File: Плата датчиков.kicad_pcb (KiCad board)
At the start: 4 copper layers, 67 x 68.5 mm, 57 parts, among them J1 A, J10 4900, J11 4900, J12 4900, J13 4900, J14 4900, J2 B, J3 C, J4 Conn_02x07_Odd_Even, J5 4900, J6 4900, J7 4900, J8 Conn_02x02_Odd_Even, J9 4900, U1 INA282, U2 INA282, U3 INA282, U4 LMV324

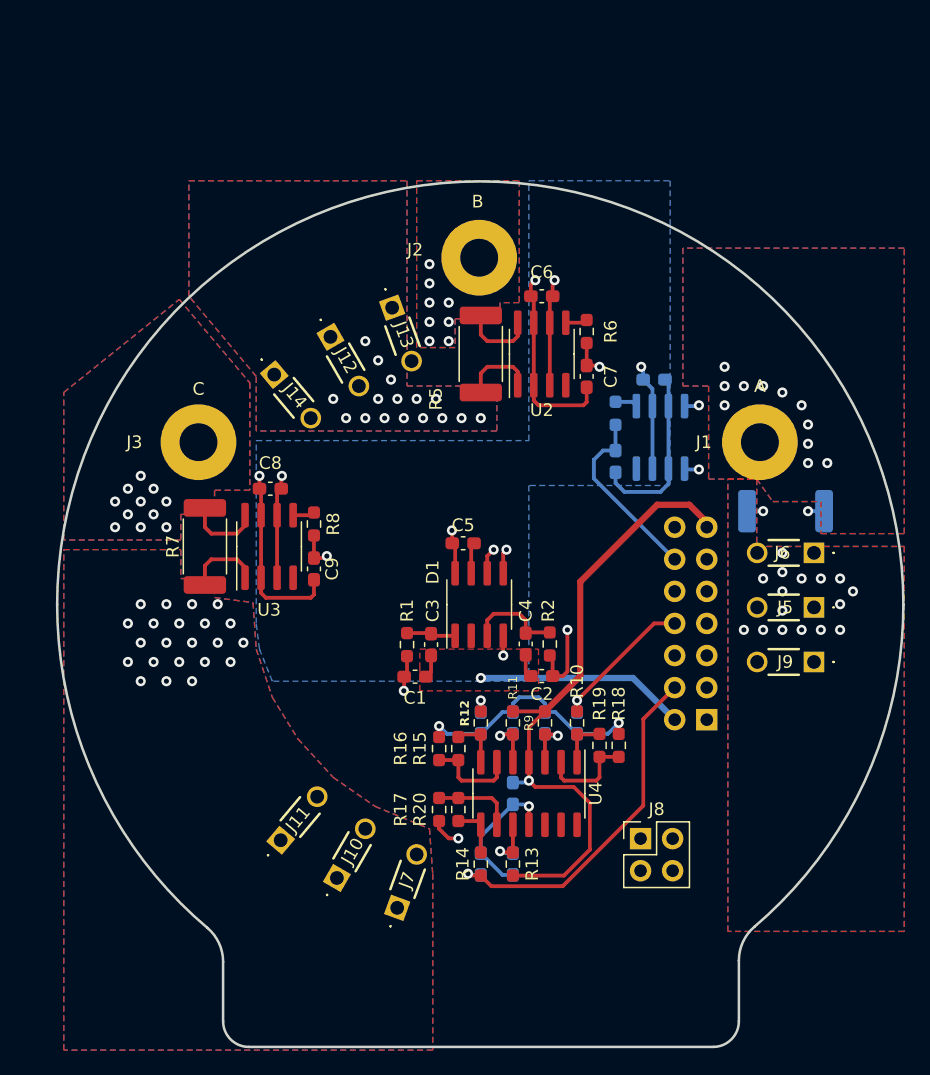
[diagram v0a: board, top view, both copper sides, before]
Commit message: VER2.0
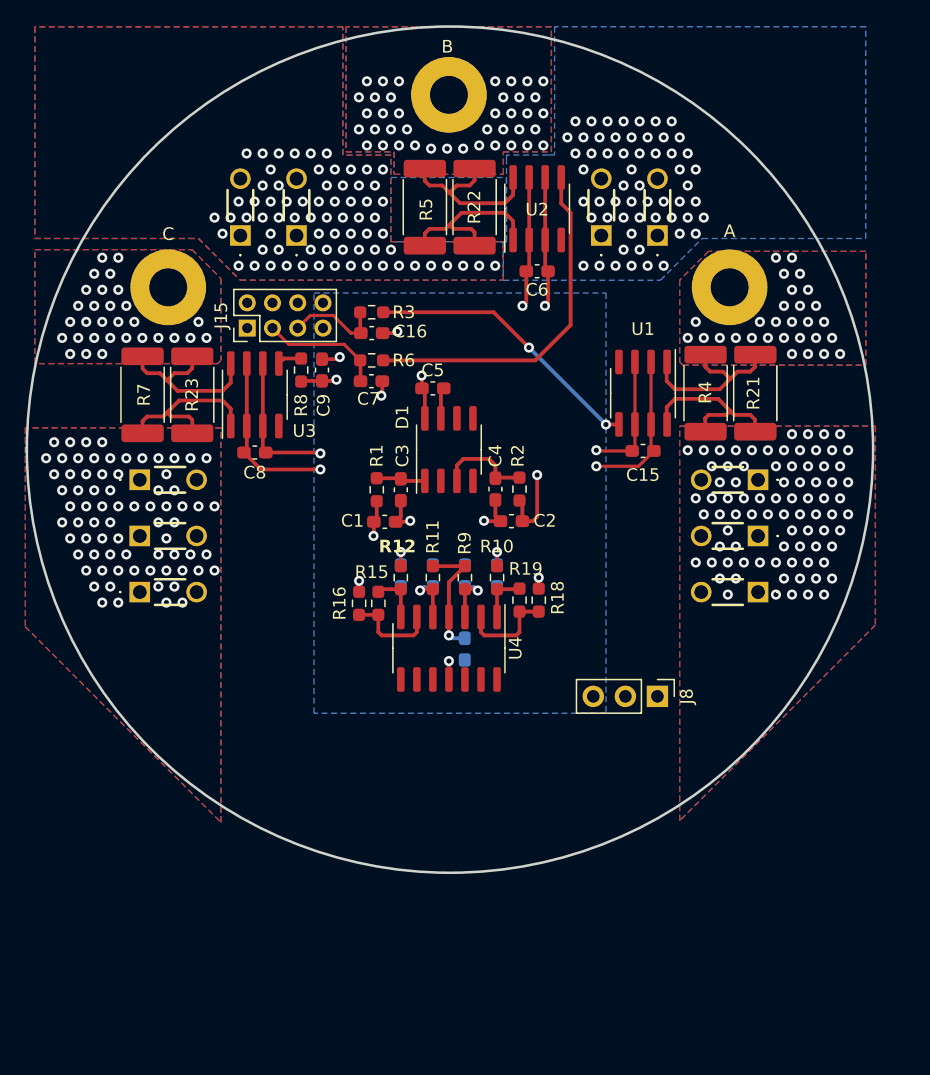
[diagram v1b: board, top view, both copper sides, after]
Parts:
- removed C14: 1u, Capacitor_SMD:C_0603_1608Metric_Pad1.08x0.95mm_HandSolder
- removed C17: 100n, Capacitor_SMD:C_0603_1608Metric_Pad1.08x0.95mm_HandSolder
- removed R13: 15k, Resistor_SMD:R_0603_1608Metric_Pad0.98x0.95mm_HandSolder
- removed R14: 120, Resistor_SMD:R_0603_1608Metric_Pad0.98x0.95mm_HandSolder
- removed R17: 1k, Resistor_SMD:R_0603_1608Metric_Pad0.98x0.95mm_HandSolder
- removed R20: 9.1k, Resistor_SMD:R_0603_1608Metric_Pad0.98x0.95mm_HandSolder
- added J15: Conn_02x04_Odd_Even, Connector_PinHeader_2.00mm:PinHeader_2x04_P2.00mm_Vertical, F.Cu at (133.4, 61.5)
- added R21: 0.5m, Resistor_SMD:R_2512_6332Metric_Pad1.40x3.35mm_HandSolder, F.Cu at (173.6, 66.6)
- added R22: 0.5m, Resistor_SMD:R_2512_6332Metric_Pad1.40x3.35mm_HandSolder, F.Cu at (151.4, 51.9)
- added R23: 0.5m, Resistor_SMD:R_2512_6332Metric_Pad1.40x3.35mm_HandSolder, F.Cu at (129.0, 66.7)
- C15, C16, R3, R4, U1: moved to F.Cu
- J4: value Conn_02x07_Odd_Even -> 4900; footprint Connector_PinSocket_2.54mm:PinSocket_2x07_P2.54mm_Vertical -> Connector_My:4900; moved to F.Cu
- J8: value Conn_02x02_Odd_Even -> Temp; footprint Connector_PinHeader_2.54mm:PinHeader_2x02_P2.54mm_Vertical -> Connector_PinHeader_2.54mm:PinHeader_1x03_P2.54mm_Vertical
- moved J4 50.2 mm to (137.3, 54.1), turned to 90 degrees
- moved J7 32.3 mm to (124.9, 82.4), turned to 0 degrees
- moved J10 31.3 mm to (124.9, 77.9), turned to 0 degrees
- moved J11 30.6 mm to (124.9, 73.5), turned to 0 degrees
- moved J12 27.1 mm to (165.9, 54.1), turned to 90 degrees
- moved C16 21.8 mm to (143.3, 61.8), turned to 0 degrees
- moved R3 20.9 mm to (143.3, 60.2), turned to 0 degrees
- moved J13 17.5 mm to (161.4, 54.1), turned to 90 degrees
- moved R6 17.2 mm to (143.3, 64.0), turned to 0 degrees
- moved C7 17.0 mm to (143.2, 65.7), turned to 0 degrees
- moved C9 15.8 mm to (139.3, 64.8), turned to 90 degrees
- moved C10 13.2 mm to (150.6, 81.1)
- moved C11 13.2 mm to (153.2, 81.1)
- moved C12 13.2 mm to (148.1, 81.1)
- moved C13 13.2 mm to (145.6, 81.1)
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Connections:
- net B renamed B+
- net C renamed C+
- net C_OUT renamed C-
- C1 pad 1: +3.3V -> +3.3VA
- C1 pad 2: GND -> GNDA
- C15 pad 1: +3.3V -> +3.3VA
- C15 pad 2: GND -> GNDA
- C16 pad 2: GND -> GNDA
- C2 pad 1: GND -> GNDA
- C3 pad 2: GND -> GNDA
- C4 pad 1: GND -> GNDA
- C5 pad 1: GND -> GNDA
- C6 pad 1: +3.3V -> +3.3VA
- C6 pad 2: GND -> GNDA
- C7 pad 2: GND -> GNDA
- C8 pad 1: +3.3V -> +3.3VA
- C8 pad 2: GND -> GNDA
- C9 pad 2: GND -> GNDA
- D1 pad 4: SCLK_MCU -> unconnected-(D1-SCLK-Pad4)
- D1 pad 5: CS_MCU -> unconnected-(D1-CS-Pad5)
- D1 pad 6: SDIO_MCU -> unconnected-(D1-SDIO-Pad6)
- D1 pad 8: GND -> GNDA
- J1 pad 1: A -> A+
- J12 pad 1: B_OUT -> B-
- J12 pad 2: B_OUT -> B-
- J13 pad 1: B_OUT -> B-
- J13 pad 2: B_OUT -> B-
- J14 pad 1: B_OUT -> B-
- J14 pad 2: B_OUT -> B-
- J4 pad 1: +3.3V -> B-
- J4 pad 2: GND -> B-
- J5 pad 1: A_OUT -> A-
- J5 pad 2: A_OUT -> A-
- J6 pad 1: A_OUT -> A-
- J6 pad 2: A_OUT -> A-
- J8 pad 2: GNDA -> PTC_Coil_B
- J8 pad 3: PTC_Coil_C -> GNDA
- J9 pad 1: A_OUT -> A-
- J9 pad 2: A_OUT -> A-
- R1 pad 1: +3.3V -> +3.3VA
- R4 pad 1: A -> A-
- R4 pad 2: A_OUT -> A+
- R5 pad 2: B_OUT -> B-
- U1 pad 1: A_OUT -> A+
- U1 pad 2: GND -> GNDA
- U1 pad 3: +3.3V -> +3.3VA
- U1 pad 6: +3.3V -> +3.3VA
- U1 pad 7: GND -> GNDA
- U1 pad 8: A -> A-
- U2 pad 1: B_OUT -> B-
- U2 pad 2: GND -> GNDA
- U2 pad 3: +3.3V -> +3.3VA
- U2 pad 6: +3.3V -> +3.3VA
- U2 pad 7: GND -> GNDA
- U3 pad 2: GND -> GNDA
- U3 pad 3: +3.3V -> +3.3VA
- U3 pad 6: +3.3V -> +3.3VA
- U3 pad 7: GND -> GNDA
- U4 pad 10: PTC_Coil_C -> unconnected-(U4C-+-Pad10)
- U4 pad 12: (no net) -> unconnected-(U4D-+-Pad12)
- U4 pad 13: (no net) -> unconnected-(U4D---Pad13)
- U4 pad 14: (no net) -> unconnected-(U4-Pad14)
- U4 pad 8: Net-(R14-Pad2) -> unconnected-(U4-Pad8)
- U4 pad 9: Net-(U4C--) -> unconnected-(U4C---Pad9)
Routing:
- net GND: track 68.2 -> 0.00 mm, vias 4 -> 0
- net +3.3V: track 46.8 -> 0.00 mm, vias 4 -> 0
- net Temp_Coil_C_MCU: track 28.4 -> 0.00 mm, vias 1 -> 0
- net Net-(R6-Pad2): track 1.74 -> 28.0 mm
- net CS_MCU: track 22.4 -> 0.00 mm, vias 1 -> 0
- net SDIO_MCU: track 22.0 -> 0.00 mm, vias 1 -> 0
- net Current_C_MCU: track 33.0 -> 11.6 mm
- net Net-(R3-Pad2): track 1.79 -> 22.3 mm, vias 0 -> 2
- net GNDA: track 33.2 -> 53.1 mm, vias 4 -> 12
- net SCLK_MCU: track 18.7 -> 0.00 mm, vias 1 -> 0
- net OUT_MCU: track 18.6 -> 36.9 mm
- net Temp_Coil_A_MCU: track 11.1 -> 29.3 mm
- net A: track 16.8 -> 0.00 mm, vias 13 -> 0
- net PTC_Coil_C: track 16.1 -> 0.00 mm, vias 1 -> 0
- net B-: track 0.00 -> 14.1 mm, vias 0 -> 128
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- added copper zone on In2.Cu, net +3.3VA
- added copper zone on B.Cu, net A+
- added copper zone on F.Cu, net A+
- added copper zone on In1.Cu, net A+
- added copper zone on In2.Cu, net A+
- added copper zone on B.Cu, net A-
- added copper zone on F.Cu, net A-
- added copper zone on In1.Cu, net A-
- added copper zone on In2.Cu, net A-
- added copper zone on B.Cu, net B-
- added copper zone on F.Cu, net B-
- added copper zone on In1.Cu, net B-
- added copper zone on In2.Cu, net B-
- added copper zone on B.Cu, net GNDA
- removed copper zone on In1.Cu, net +3.3V
- removed copper zone on B.Cu, net A
- removed copper zone on F.Cu, net A
- removed copper zone on In1.Cu, net A
- removed copper zone on In2.Cu, net A
- removed copper zone on B.Cu, net A_OUT
- removed copper zone on F.Cu, net A_OUT
- removed copper zone on In1.Cu, net A_OUT
- removed copper zone on In2.Cu, net A_OUT
- removed copper zone on B.Cu, net B_OUT
- removed copper zone on F.Cu, net B_OUT
- removed copper zone on In1.Cu, net B_OUT
- removed copper zone on In2.Cu, net B_OUT
- removed copper zone on B.Cu, net GND
- removed copper zone on F.Cu, net GND
- removed copper zone on In2.Cu, net GNDA
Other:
- board size 67 x 68.5 mm -> 67 x 67 mm
